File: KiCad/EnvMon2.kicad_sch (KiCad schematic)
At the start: 32 parts, among them J1 USB-C, J2 DC, J3 TEMP, M1 OLED1.5-RGB, U1 LMR16006+FB, U2 SCD41, U3 FT231XQ, U4 ESP32-PICO-MINI-02, U5 QR

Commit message: Tidy
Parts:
- D2: footprint Diode_SMD:D_1206_3216Metric -> RevK:D_1206
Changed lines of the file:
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@@
     (property "Reference" "D2" (id 0) (at 83.185 22.4282 0))
     (property "Value" "D" (id 1) (at 83.185 24.7396 0))
-    (property "Footprint" "Diode_SMD:D_1206_3216Metric" (id 2) (at 83.185 27.94 0)
+    (property "Footprint" "RevK:D_1206" (id 2) (at 83.185 27.94 0)
       (effects (font (size 1.27 1.27)) hide)
     )
@@
     )
     (path "/bbc62690-b8fb-438a-8ee0-c77d65956f89"
-      (reference "D2") (unit 1) (value "D") (footprint "Diode_SMD:D_1206_3216Metric")
+      (reference "D2") (unit 1) (value "D") (footprint "RevK:D_1206")
     )
     (path "/00000000-0000-0000-0000-000060cf36bc"

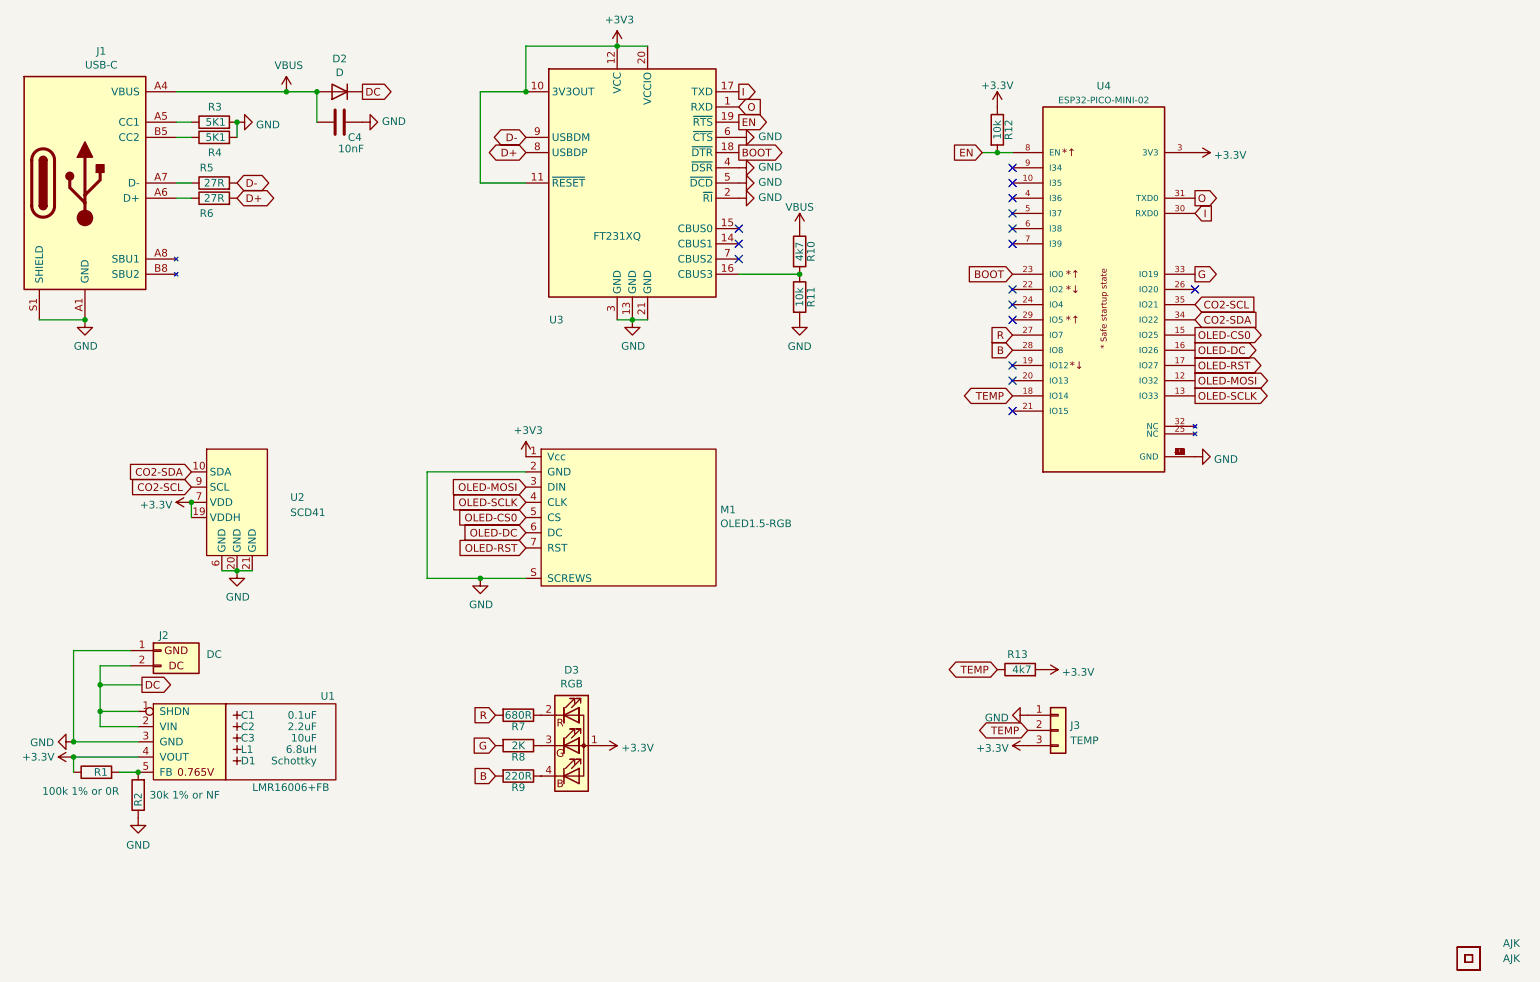
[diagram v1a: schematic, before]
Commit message: Tidy
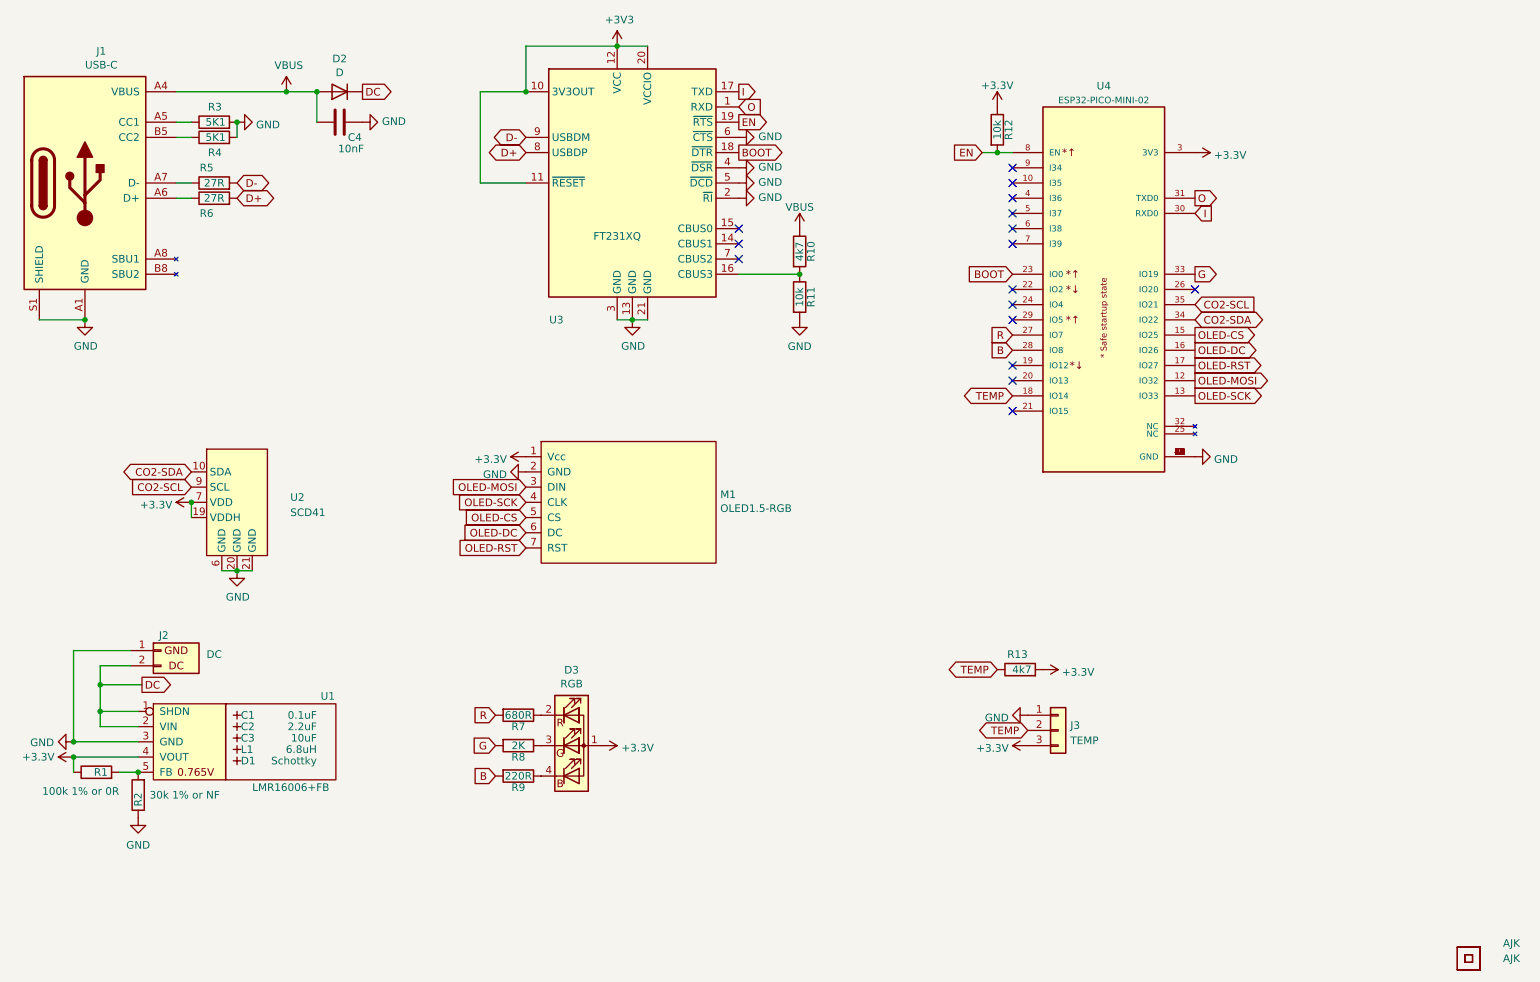
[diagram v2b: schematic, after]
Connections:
- net GND: no longer M1.S (SCREWS)
- net OLED-CS0 renamed OLED-CS
- net OLED-SCLK renamed OLED-SCK
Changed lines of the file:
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@@
   (junction (at 43.18 127) (diameter 0) (color 0 0 0 0)
-  )
-  (junction (at 106.68 109.22) (diameter 0) (color 0 0 0 0)
   )
   (junction (at 49.53 141.605) (diameter 0) (color 0 0 0 0)
@@
     (stroke (width 0) (type default) (color 0 0 0 0))
   )
-  (wire (pts (xy 97.79 109.22) (xy 106.68 109.22))
-    (stroke (width 0) (type default) (color 0 0 0 0))
-  )
   (wire (pts (xy 66.04 33.02) (xy 66.04 35.56))
     (stroke (width 0) (type default) (color 0 0 0 0))
@@
     (stroke (width 0) (type default) (color 0 0 0 0))
   )
-  (wire (pts (xy 97.79 91.44) (xy 97.79 109.22))
-    (stroke (width 0) (type default) (color 0 0 0 0))
-  )
   (wire (pts (xy 106.68 27.94) (xy 106.68 43.18))
     (stroke (width 0) (type default) (color 0 0 0 0))
@@
     (stroke (width 0) (type default) (color 0 0 0 0))
   )
-  (wire (pts (xy 97.79 91.44) (xy 114.3 91.44))
-    (stroke (width 0) (type default) (color 0 0 0 0))
-  )
   (wire (pts (xy 193.04 38.1) (xy 195.58 38.1))
     (stroke (width 0) (type default) (color 0 0 0 0))
@@
   )
   (wire (pts (xy 66.04 107.95) (xy 68.58 107.95))
-    (stroke (width 0) (type default) (color 0 0 0 0))
-  )
-  (wire (pts (xy 114.3 109.22) (xy 106.68 109.22))
     (stroke (width 0) (type default) (color 0 0 0 0))
   )
@@
     )
   )
-  (global_label "OLED-SCLK" (shape output) (at 226.06 78.74 0) (fields_autoplaced)
-    (effects (font (size 1.27 1.27)) (justify left))
-    (property "Intersheet References" "${INTERSHEET_REFS}" (id 0) (at 239.5118 78.6606 0)
-      (effects (font (size 1.27 1.27)) (justify left) hide)
-    )
-  )
-  (global_label "OLED-CS0" (shape output) (at 226.06 68.58 0) (fields_autoplaced)
-    (effects (font (size 1.27 1.27)) (justify left))
-    (property "Intersheet References" "${INTERSHEET_REFS}" (id 0) (at 238.4232 68.5006 0)
-      (effects (font (size 1.27 1.27)) (justify left) hide)
-    )
-  )
-  (global_label "OLED-SCLK" (shape input) (at 114.3 96.52 180) (fields_autoplaced)
-    (effects (font (size 1.27 1.27)) (justify right))
-    (property "Intersheet References" "${INTERSHEET_REFS}" (id 0) (at 4.445 -33.655 0)
-      (effects (font (size 1.27 1.27)) hide)
+  (global_label "OLED-SCK" (shape output) (at 226.06 78.74 0) (fields_autoplaced)
+    (effects (font (size 1.27 1.27)) (justify left))
+    (property "Intersheet References" "${INTERSHEET_REFS}" (id 0) (at 238.4837 78.6606 0)
+      (effects (font (size 1.27 1.27)) (justify left) hide)
+    )
+  )
+  (global_label "OLED-CS" (shape output) (at 226.06 68.58 0) (fields_autoplaced)
+    (effects (font (size 1.27 1.27)) (justify left))
+    (property "Intersheet References" "${INTERSHEET_REFS}" (id 0) (at 237.2137 68.5006 0)
+      (effects (font (size 1.27 1.27)) (justify left) hide)
+    )
+  )
+  (global_label "OLED-SCK" (shape input) (at 114.3 96.52 180) (fields_autoplaced)
+    (effects (font (size 1.27 1.27)) (justify right))
+    (property "Intersheet References" "${INTERSHEET_REFS}" (id 0) (at 101.8763 96.4406 0)
+      (effects (font (size 1.27 1.27)) (justify right) hide)
     )
   )
@@
     )
   )
-  (global_label "CO2-SDA" (shape input) (at 226.06 66.04 0) (fields_autoplaced)
-    (effects (font (size 1.27 1.27)) (justify left))
-    (property "Intersheet References" "${INTERSHEET_REFS}" (id 0) (at 274.955 189.865 0)
-      (effects (font (size 1.27 1.27)) hide)
+  (global_label "CO2-SDA" (shape bidirectional) (at 226.06 66.04 0) (fields_autoplaced)
+    (effects (font (size 1.27 1.27)) (justify left))
+    (property "Intersheet References" "${INTERSHEET_REFS}" (id 0) (at 237.3347 65.9606 0)
+      (effects (font (size 1.27 1.27)) (justify left) hide)
     )
   )
@@
     )
   )
-  (global_label "CO2-SDA" (shape input) (at 58.42 91.44 180) (fields_autoplaced)
-    (effects (font (size 1.27 1.27)) (justify right))
-    (property "Intersheet References" "${INTERSHEET_REFS}" (id 0) (at 9.525 -32.385 0)
-      (effects (font (size 1.27 1.27)) hide)
+  (global_label "CO2-SDA" (shape bidirectional) (at 58.42 91.44 180) (fields_autoplaced)
+    (effects (font (size 1.27 1.27)) (justify right))
+    (property "Intersheet References" "${INTERSHEET_REFS}" (id 0) (at 47.1453 91.3606 0)
+      (effects (font (size 1.27 1.27)) (justify right) hide)
     )
   )
@@
     )
   )
-  (global_label "OLED-CS0" (shape input) (at 114.3 99.06 180) (fields_autoplaced)
-    (effects (font (size 1.27 1.27)) (justify right))
-    (property "Intersheet References" "${INTERSHEET_REFS}" (id 0) (at 4.445 -33.655 0)
-      (effects (font (size 1.27 1.27)) hide)
+  (global_label "OLED-CS" (shape input) (at 114.3 99.06 180) (fields_autoplaced)
+    (effects (font (size 1.27 1.27)) (justify right))
+    (property "Intersheet References" "${INTERSHEET_REFS}" (id 0) (at 103.1463 98.9806 0)
+      (effects (font (size 1.27 1.27)) (justify right) hide)
     )
   )
@@
     (pin "1")
   )
-  (symbol (lib_id "power:GND") (at 106.68 109.22 0) (unit 1)
-    (in_bom yes) (on_board yes)
-    (property "Reference" "#PWR010" (id 0) (at 106.68 115.57 0)
-      (effects (font (size 1.27 1.27)) hide)
-    )
-    (property "Value" "GND" (id 1) (at 106.807 113.6142 0))
-    (property "Footprint" "" (id 2) (at 106.68 109.22 0)
-      (effects (font (size 1.27 1.27)) hide)
-    )
-    (property "Datasheet" "" (id 3) (at 106.68 109.22 0)
-      (effects (font (size 1.27 1.27)) hide)
-    )
-    (pin "1")
-  )
   (symbol (lib_id "power:GND") (at 66.04 107.95 0) (unit 1)
     (in_bom yes) (on_board yes)
@@
     (pin "2")
   )
-  (symbol (lib_id "power:+3V3") (at 114.3 88.9 0) (unit 1)
-    (in_bom yes) (on_board yes)
-    (property "Reference" "#PWR011" (id 0) (at 114.3 92.71 0)
-      (effects (font (size 1.27 1.27)) hide)
-    )
-    (property "Value" "+3V3" (id 1) (at 114.681 84.5058 0))
-    (property "Footprint" "" (id 2) (at 114.3 88.9 0)
-      (effects (font (size 1.27 1.27)) hide)
-    )
-    (property "Datasheet" "" (id 3) (at 114.3 88.9 0)
-      (effects (font (size 1.27 1.27)) hide)
-    )
-    (pin "1")
-  )
-  (symbol (lib_id "RevK:OLED1.5-RGB") (at 114.3 88.9 0) (unit 1)
+  (symbol (lib_id "RevK:OLED1.5-RGB") (at 114.3 86.36 0) (unit 1)
     (in_bom no) (on_board yes)
-    (property "Reference" "M1" (id 0) (at 146.7612 97.7646 0)
-      (effects (font (size 1.27 1.27)) (justify left))
-    )
-    (property "Value" "OLED1.5-RGB" (id 1) (at 146.7612 100.076 0)
-      (effects (font (size 1.27 1.27)) (justify left))
-    )
-    (property "Footprint" "RevK:OLED1.5-RGB" (id 2) (at 133.35 111.76 0)
-      (effects (font (size 1.27 1.27)) hide)
-    )
-    (property "Datasheet" "" (id 3) (at 114.3 86.36 0)
+    (property "Reference" "M1" (id 0) (at 146.7612 95.2246 0)
+      (effects (font (size 1.27 1.27)) (justify left))
+    )
+    (property "Value" "OLED1.5-RGB" (id 1) (at 146.7612 97.536 0)
+      (effects (font (size 1.27 1.27)) (justify left))
+    )
+    (property "Footprint" "RevK:OLED1.5-RGB" (id 2) (at 133.35 109.22 0)
+      (effects (font (size 1.27 1.27)) hide)
+    )
+    (property "Datasheet" "" (id 3) (at 114.3 83.82 0)
       (effects (font (size 1.27 1.27)) hide)
     )
@@
     (pin "6")
     (pin "7")
-    (pin "S")
   )
   (symbol (lib_id "RevK:AJK") (at 276.86 172.72 0) (unit 1)
@@
     (pin "1")
   )
+  (symbol (lib_id "power:GND") (at 114.3 91.44 270) (unit 1)
+    (in_bom yes) (on_board yes) (fields_autoplaced)
+    (property "Reference" "#PWR?" (id 0) (at 107.95 91.44 0)
+      (effects (font (size 1.27 1.27)) hide)
+    )
+    (property "Value" "GND" (id 1) (at 111.1251 91.8738 90)
+      (effects (font (size 1.27 1.27)) (justify right))
+    )
+    (property "Footprint" "" (id 2) (at 114.3 91.44 0)
+      (effects (font (size 1.27 1.27)) hide)
+    )
+    (property "Datasheet" "" (id 3) (at 114.3 91.44 0)
+      (effects (font (size 1.27 1.27)) hide)
+    )
+    (pin "1")
+  )
   (symbol (lib_id "power:GND") (at 198.12 132.08 270) (unit 1)
     (in_bom yes) (on_board yes) (fields_autoplaced)
@@
     )
     (property "Datasheet" "" (id 3) (at 58.42 96.52 0)
+      (effects (font (size 1.27 1.27)) hide)
+    )
+    (pin "1")
+  )
+  (symbol (lib_id "power:+3.3V") (at 114.3 88.9 90) (unit 1)
+    (in_bom yes) (on_board yes) (fields_autoplaced)
+    (property "Reference" "#PWR?" (id 0) (at 118.11 88.9 0)
+      (effects (font (size 1.27 1.27)) hide)
+    )
+    (property "Value" "+3.3V" (id 1) (at 111.125 89.3338 90)
+      (effects (font (size 1.27 1.27)) (justify left))
+    )
+    (property "Footprint" "" (id 2) (at 114.3 88.9 0)
+      (effects (font (size 1.27 1.27)) hide)
+    )
+    (property "Datasheet" "" (id 3) (at 114.3 88.9 0)
       (effects (font (size 1.27 1.27)) hide)
     )
@@
       (reference "#PWR09") (unit 1) (value "GND") (footprint "")
     )
-    (path "/00000000-0000-0000-0000-00006048883f"
-      (reference "#PWR010") (unit 1) (value "GND") (footprint "")
-    )
-    (path "/00000000-0000-0000-0000-0000604b79ca"
-      (reference "#PWR011") (unit 1) (value "+3V3") (footprint "")
-    )
     (path "/00000000-0000-0000-0000-000060a44fe5"
       (reference "#PWR012") (unit 1) (value "+3.3V") (footprint "")
@@
       (reference "#PWR026") (unit 1) (value "GND") (footprint "")
     )
+    (path "/08af68ca-feb6-4d9f-97d4-c810080fe2bb"
+      (reference "#PWR?") (unit 1) (value "GND") (footprint "")
+    )
+    (path "/302ce8d8-fad8-4e86-ae09-959aa671fce0"
+      (reference "#PWR?") (unit 1) (value "+3.3V") (footprint "")
+    )
     (path "/00000000-0000-0000-0000-0000610f9b88"
